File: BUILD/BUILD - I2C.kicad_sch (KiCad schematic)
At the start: 32 parts, among them J1-INPUT1 AudioJack3, J1-OUTPUT AudioJack3, SW1 SW_Push, SW2 SW_Push, SW3 SW_DIP_x04, SW4 SW_Push, SW5-F1 SW_Push, SW6-F2 SW_Push, SW7-F3 SW_Push, SW8-F4 SW_Push, SW9-F5 SW_Push, U1 LM386

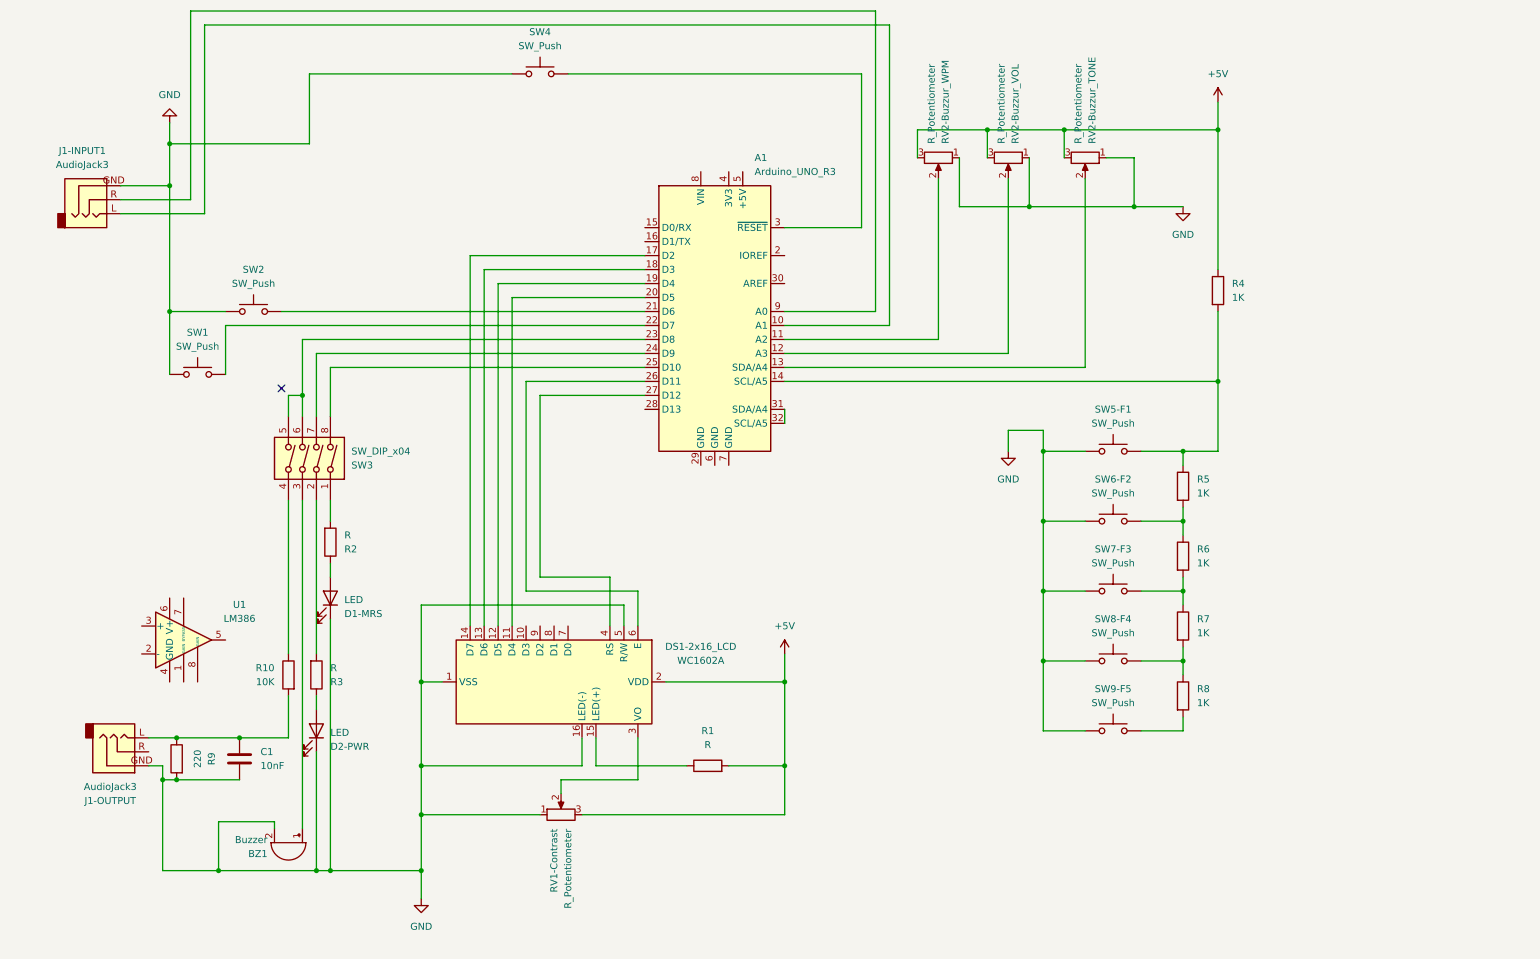
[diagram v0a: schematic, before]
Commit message: 2025-06-19-01
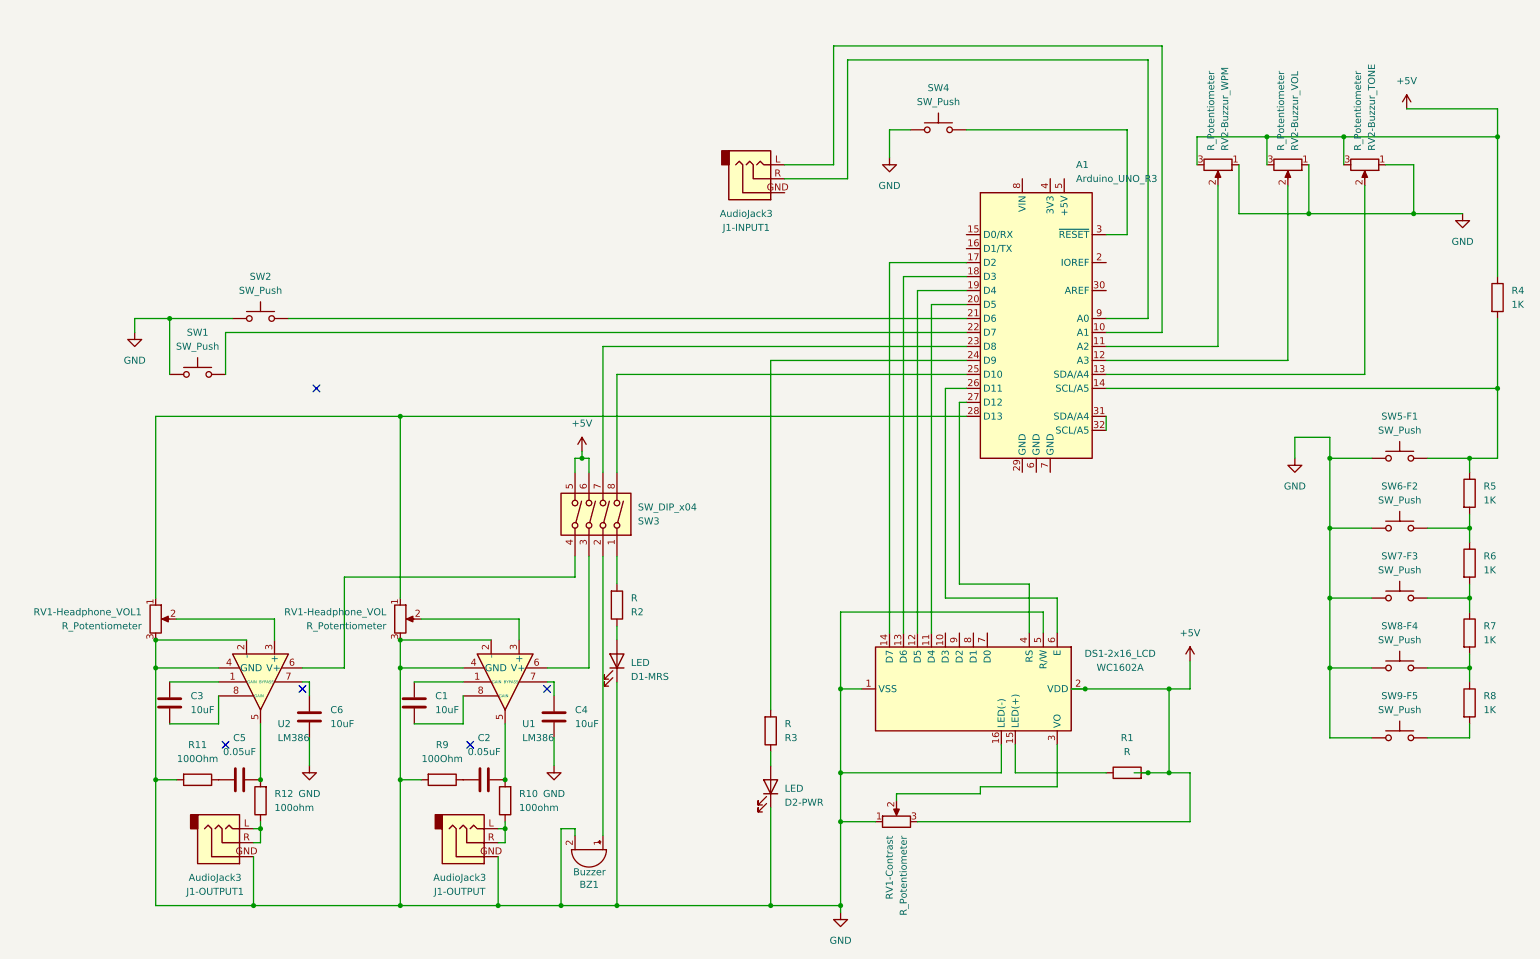
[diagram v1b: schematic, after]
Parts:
- added C2, C5: 0.05uF, symbol Device:C
- added C3, C4, C6: 10uF, symbol Device:C
- added J1-OUTPUT1: AudioJack3, symbol Connector_Audio:AudioJack3
- added R11: 100Ohm, symbol Device:R
- added R12: 100ohm, symbol Device:R
- added RV1-Headphone_VOL, RV1-Headphone_VOL1: R_Potentiometer, symbol Device:R_Potentiometer
- added U2: LM386, symbol Amplifier_Audio:LM386
- C1: value 10nF -> 10uF
- R10: value 10K -> 100ohm
- R9: value 220 -> 100Ohm
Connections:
- net +5V: now also SW3.5, SW3.6
- net GND: now also U1.2 (-), U1.4 (GND), C4.2, C6.2, J1-OUTPUT1.GND, R11.2, RV1-Headphone_VOL.3, RV1-Headphone_VOL1.3, U2.2 (-), U2.4 (GND); no longer C1.2, J1-INPUT1.GND
- net at R3.2: now also A1.24 (D9); no longer SW3.2
- net at SW3.7: now also A1.23 (D8); no longer A1.24 (D9)
- net at A1.28 (D13): now also RV1-Headphone_VOL.1, RV1-Headphone_VOL1.1
- net at J1-OUTPUT.R: now also J1-OUTPUT.L, R10.1
- net at U1.1 (GAIN): now also C1.1
- net at U1.3 (+): now also RV1-Headphone_VOL.2
- net at U1.5: now also R10.2, C2.1
- net at U1.6 (V+): now also SW3.3
- net at U1.7 (BYPASS): now also C4.1
- net at U1.8 (GAIN): now also C1.2
- net at BZ1.1 (+): now also SW3.2; no longer SW3.3
- net at SW3.4: now also U2.6 (V+); no longer R10.1
- new net: C2.2, R9.1
- new net: J1-OUTPUT1.L, J1-OUTPUT1.R, R12.1
- new net: C5.1, R12.2, U2.5
- new net: C5.2, R11.1
- new net: C6.1, U2.7 (BYPASS)
- new net: C3.1, U2.1 (GAIN)
- new net: C3.2, U2.8 (GAIN)
- new net: RV1-Headphone_VOL1.2, U2.3 (+)
- no-connect marks 1 -> 5
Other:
- moved on the sheet: A1, BZ1, D1-MRS, D2-PWR, DS1-2x16_LCD, J1-INPUT1, J1-OUTPUT, R1, R2, R3, R4, R5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
